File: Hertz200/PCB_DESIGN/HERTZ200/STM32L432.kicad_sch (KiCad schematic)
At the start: 10 parts

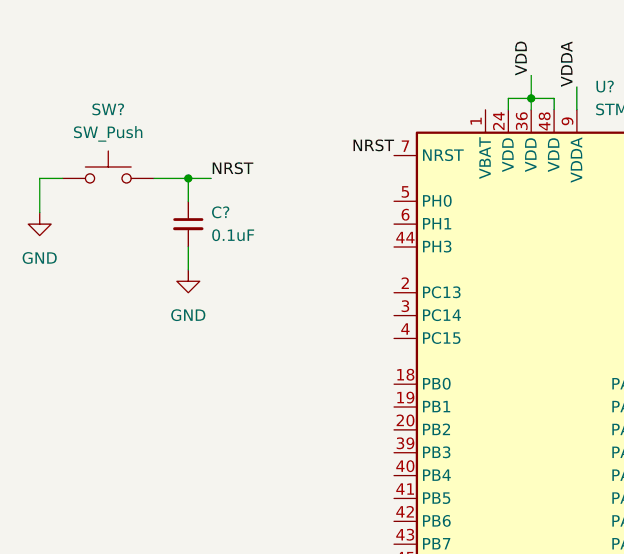
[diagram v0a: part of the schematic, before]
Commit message: schematics_Power_section
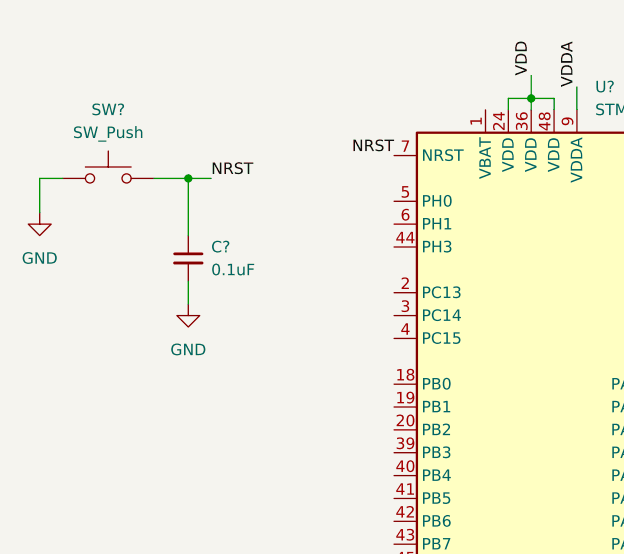
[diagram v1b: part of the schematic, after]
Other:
- moved on the sheet: C?
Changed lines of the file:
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@@
     (stroke (width 0) (type default) (color 0 0 0 0))
   )
-  (wire (pts (xy 96.52 71.12) (xy 96.52 73.66))
+  (wire (pts (xy 96.52 74.93) (xy 96.52 77.47))
     (stroke (width 0) (type default) (color 0 0 0 0))
   )
@@
     (stroke (width 0) (type default) (color 0 0 0 0))
   )
-  (wire (pts (xy 96.52 63.5) (xy 96.52 66.04))
+  (wire (pts (xy 96.52 63.5) (xy 96.52 69.85))
     (stroke (width 0) (type default) (color 0 0 0 0))
   )
@@
     (pin "1")
   )
-  (symbol (lib_id "power:GND") (at 96.52 73.66 0) (unit 1)
-    (in_bom yes) (on_board yes) (fields_autoplaced)
-    (property "Reference" "#PWR?" (id 0) (at 96.52 80.01 0)
-      (effects (font (size 1.27 1.27)) hide)
-    )
-    (property "Value" "GND" (id 1) (at 96.52 78.74 0))
-    (property "Footprint" "" (id 2) (at 96.52 73.66 0)
-      (effects (font (size 1.27 1.27)) hide)
-    )
-    (property "Datasheet" "" (id 3) (at 96.52 73.66 0)
+  (symbol (lib_id "power:GND") (at 96.52 77.47 0) (unit 1)
+    (in_bom yes) (on_board yes) (fields_autoplaced)
+    (property "Reference" "#PWR?" (id 0) (at 96.52 83.82 0)
+      (effects (font (size 1.27 1.27)) hide)
+    )
+    (property "Value" "GND" (id 1) (at 96.52 82.55 0))
+    (property "Footprint" "" (id 2) (at 96.52 77.47 0)
+      (effects (font (size 1.27 1.27)) hide)
+    )
+    (property "Datasheet" "" (id 3) (at 96.52 77.47 0)
       (effects (font (size 1.27 1.27)) hide)
     )
@@
     (pin "2")
   )
-  (symbol (lib_id "Device:C_Small") (at 96.52 68.58 0) (unit 1)
-    (in_bom yes) (on_board yes) (fields_autoplaced)
-    (property "Reference" "C?" (id 0) (at 99.06 67.3162 0)
-      (effects (font (size 1.27 1.27)) (justify left))
-    )
-    (property "Value" "0.1uF" (id 1) (at 99.06 69.8562 0)
-      (effects (font (size 1.27 1.27)) (justify left))
-    )
-    (property "Footprint" "" (id 2) (at 96.52 68.58 0)
-      (effects (font (size 1.27 1.27)) hide)
-    )
-    (property "Datasheet" "~" (id 3) (at 96.52 68.58 0)
-      (effects (font (size 1.27 1.27)) hide)
-    )
+  (symbol (lib_id "Device:C_Small") (at 96.52 72.39 0) (unit 1)
+    (in_bom yes) (on_board yes) (fields_autoplaced)
+    (property "Reference" "C?" (id 0) (at 99.06 71.1262 0)
+      (effects (font (size 1.27 1.27)) (justify left))
+    )
+    (property "Value" "0.1uF" (id 1) (at 99.06 73.6662 0)
+      (effects (font (size 1.27 1.27)) (justify left))
+    )
+    (property "Footprint" "" (id 2) (at 96.52 72.39 0)
+      (effects (font (size 1.27 1.27)) hide)
+    )
+    (property "Datasheet" "~" (id 3) (at 96.52 72.39 0)
+      (effects (font (size 1.27 1.27)) hide)
+    )
